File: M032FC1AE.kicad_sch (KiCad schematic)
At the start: 21 parts, among them IC1 M032FC1AE, J1 Conn_01x10, J2 Conn_01x03, J3 Conn_01x04, Q1 S8050, SW1 SW_Push, SW2 SW_Slide_DPDT, U1 AMS1117-1.8, U2 AMS1117-3.3

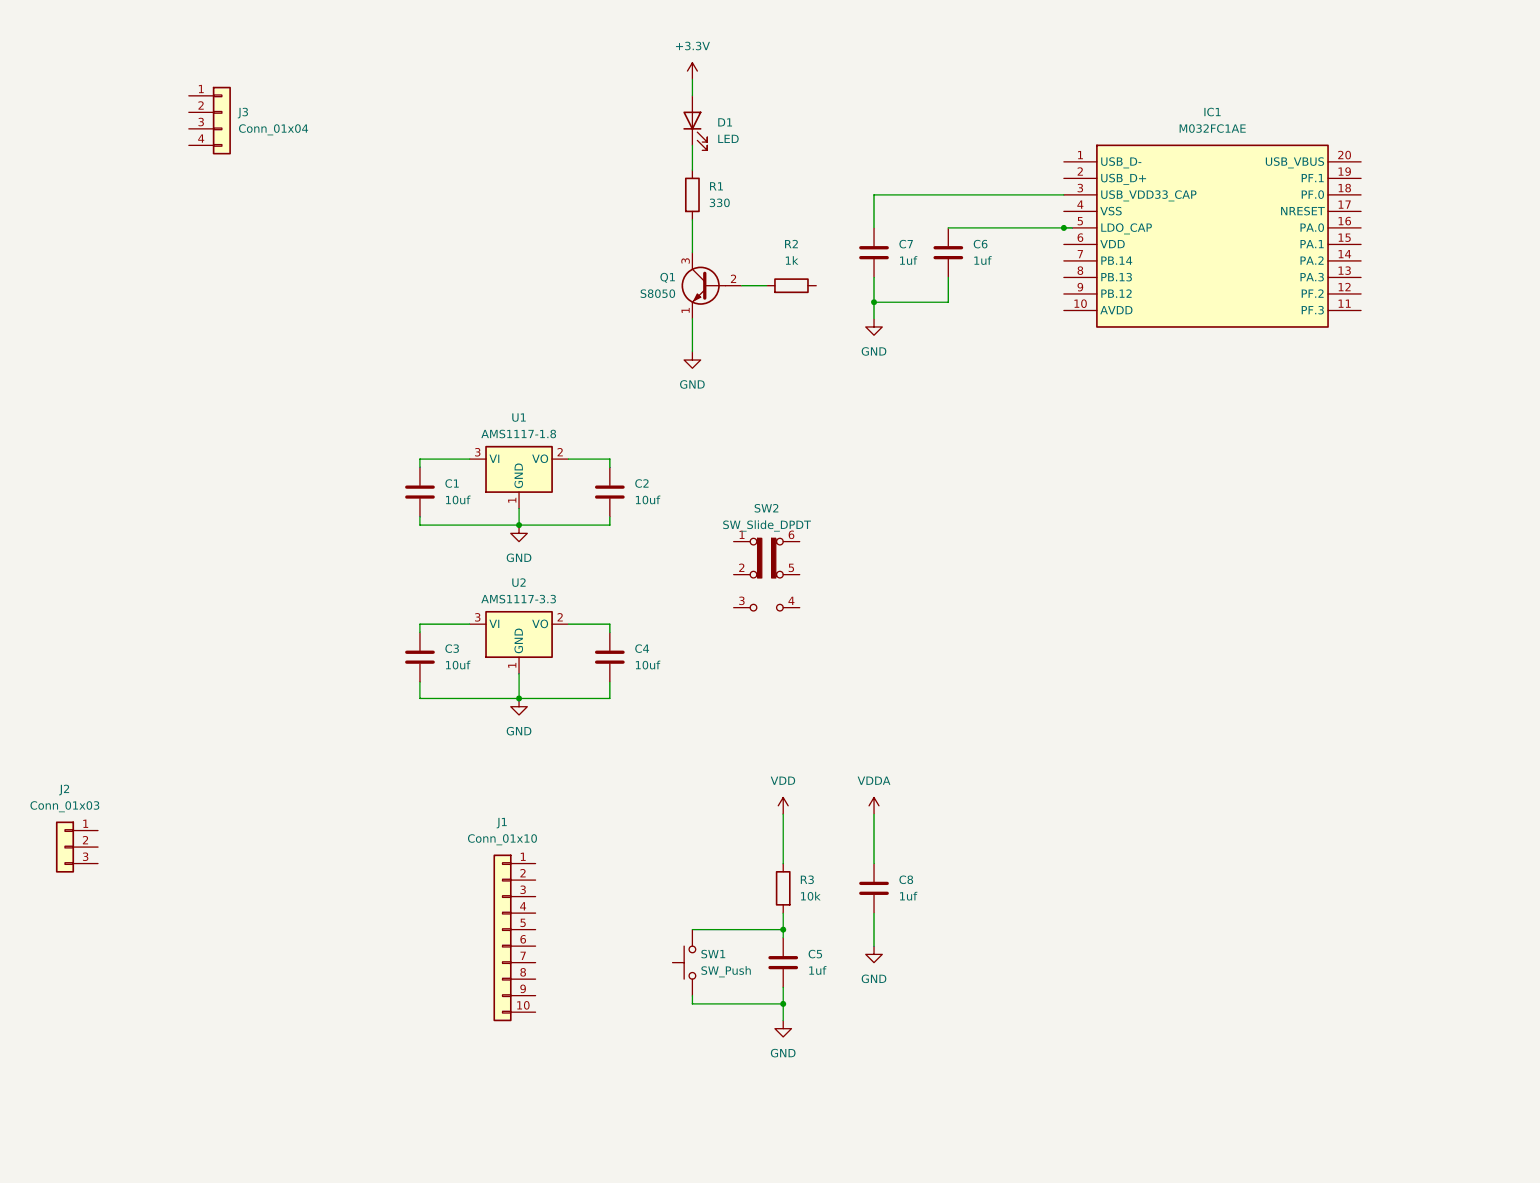
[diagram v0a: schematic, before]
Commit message: fff
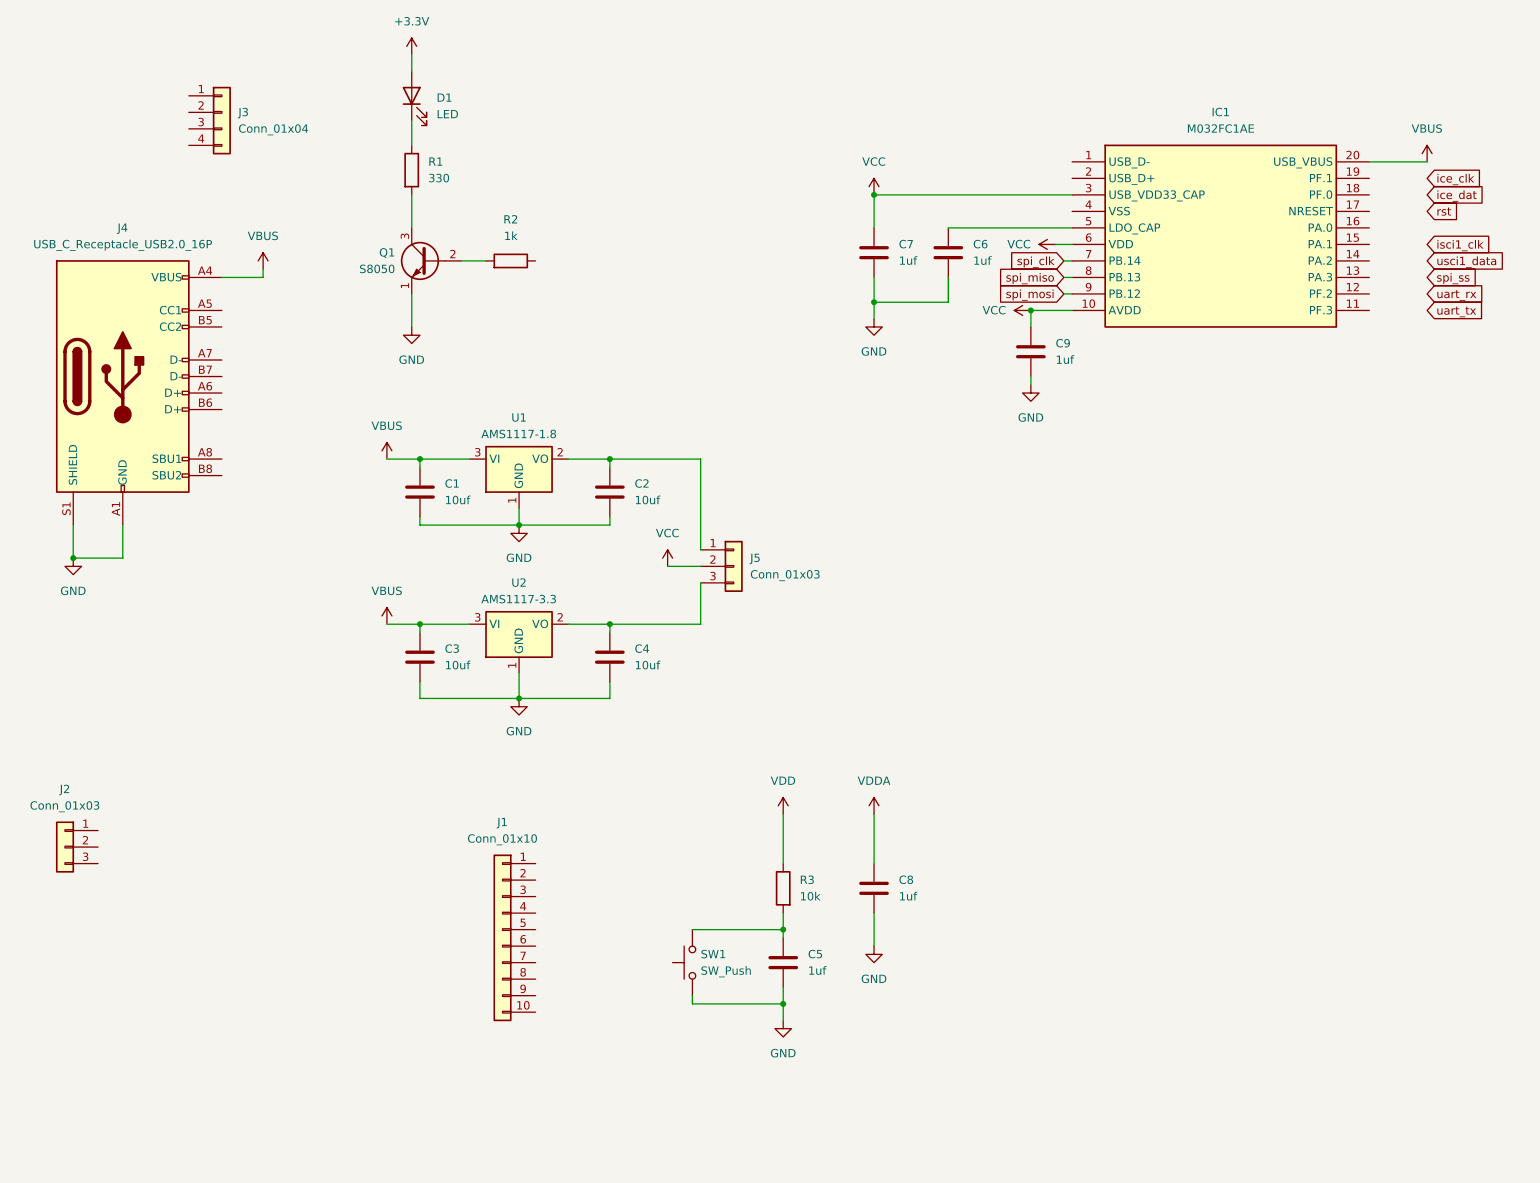
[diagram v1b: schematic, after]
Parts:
- removed SW2: SW_Slide_DPDT, Button_Switch_THT:SW_E-Switch_EG2219_DPDT_Angled, symbol Switch:SW_Slide_DPDT
- added C9: 1uf, Capacitor_SMD:C_0603_1608Metric_Pad1.08x0.95mm_HandSolder, symbol Device:C
- added J4: USB_C_Receptacle_USB2.0_16P, symbol Connector:USB_C_Receptacle_USB2.0_16P
- added J5: Conn_01x03, symbol Connector_Generic:Conn_01x03
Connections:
- net GND: now also C9.2, J4.A1 (GND), J4.A12 (GND), J4.B1 (GND), J4.B12 (GND), J4.S1 (SHIELD)
- net VBUS: now reaches C3.1, U2.3 (VI)
- net VBUS: now also C1.1, IC1.20 (USB_VBUS), U1.3 (VI), J4.A4 (VBUS), J4.A9 (VBUS), J4.B4 (VBUS), J4.B9 (VBUS)
- net at C4.1, U2.2 (VO): now also J5.3 (Pin_3)
- net VCC: now reaches IC1.10 (AVDD)
- net VCC: now also C7.1, IC1.3 (USB_VDD33_CAP), IC1.6 (VDD), C9.1, J5.2 (Pin_2)
- net spi_clk: now reaches IC1.7 (PB.14)
- net spi_miso: now reaches IC1.8 (PB.13)
- net spi_mosi: now reaches IC1.9 (PB.12)
- net at C2.1, U1.2 (VO): now also J5.1 (Pin_1)
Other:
- moved on the sheet: D1, IC1, Q1, R1, R2

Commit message: ddd
Change-Id: I6d4370392eb8b31b3cfbca76c540ab61eec68797
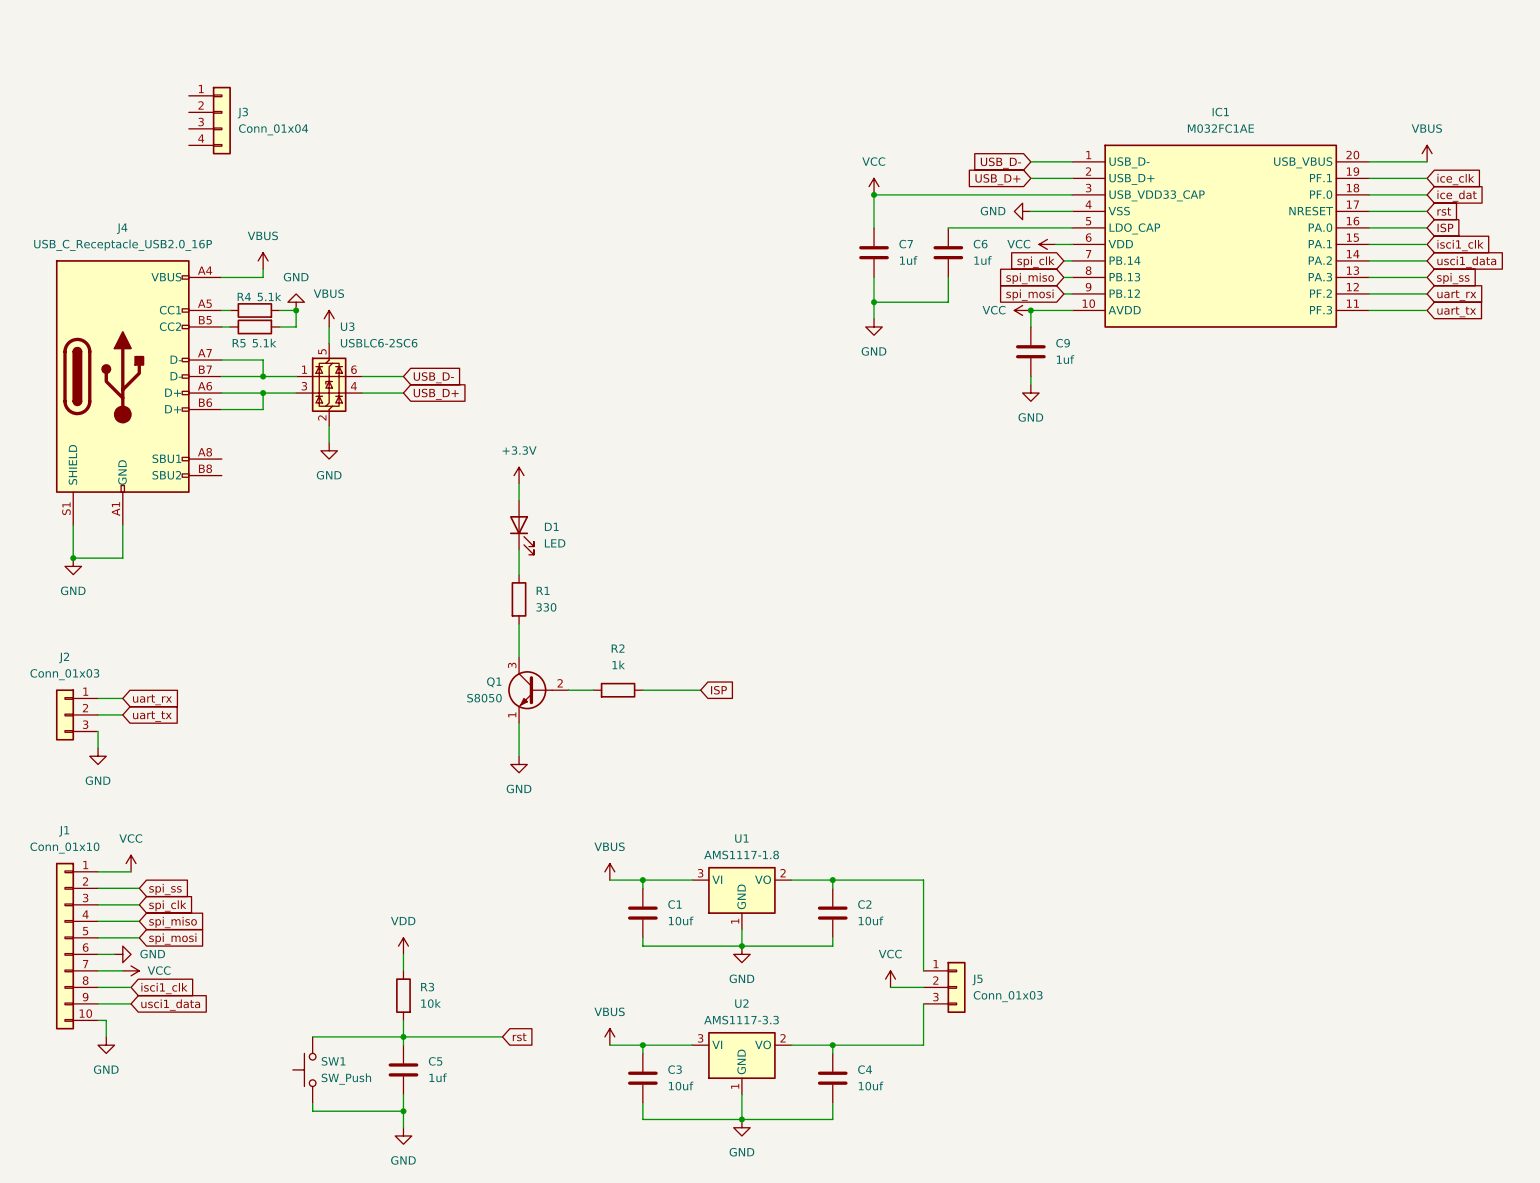
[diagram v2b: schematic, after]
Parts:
- removed C8: 1uf, Capacitor_SMD:C_0603_1608Metric_Pad1.08x0.95mm_HandSolder, symbol Device:C
- added R4, R5: 5.1k, Resistor_SMD:R_0603_1608Metric_Pad0.98x0.95mm_HandSolder, symbol Device:R
- added U3: USBLC6-2SC6, Package_TO_SOT_SMD:SOT-23-6, symbol Power_Protection:USBLC6-2SC6
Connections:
- net GND: now also IC1.4 (VSS), J1.10 (Pin_10), J1.6 (Pin_6), J2.3 (Pin_3), R4.2, R5.2, U3.2 (GND)
- net VBUS: now also U3.5 (VBUS)
- net VCC: now also J1.1 (Pin_1), J1.7 (Pin_7)
- net ice_clk: now also IC1.19 (PF.1)
- net ice_dat: now also IC1.18 (PF.0)
- net isci1_clk: now also IC1.15 (PA.1), J1.8 (Pin_8)
- net rst: now also C5.1, IC1.17 (NRESET), R3.2, SW1.2
- net spi_clk: now also J1.3 (Pin_3)
- net spi_miso: now also J1.4 (Pin_4)
- net spi_mosi: now also J1.5 (Pin_5)
- net spi_ss: now also IC1.13 (PA.3), J1.2 (Pin_2)
- net uart_rx: now also IC1.12 (PF.2), J2.1 (Pin_1)
- net uart_tx: now also IC1.11 (PF.3), J2.2 (Pin_2)
- net usci1_data: now also IC1.14 (PA.2), J1.9 (Pin_9)
- net ISP: now reaches R2.1
- net ISP: now also IC1.16 (PA.0)
- net USB_D-: now reaches IC1.1 (USB_D-)
- net USB_D-: now also U3.6 (I/O1)
- net USB_D+: now reaches IC1.2 (USB_D+)
- net USB_D+: now also U3.4 (I/O2)
- net at J4.A5 (CC1): now also R4.1
- net at J4.A6 (D+): now also J4.B6 (D+), U3.3 (I/O2)
- net at J4.A7 (D-): now also J4.B7 (D-), U3.1 (I/O1)
- net at J4.B5 (CC2): now also R5.1
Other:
- moved on the sheet: C1, C2, C3, C4, C5, D1, J1, J2, J5, Q1, R1, R2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
